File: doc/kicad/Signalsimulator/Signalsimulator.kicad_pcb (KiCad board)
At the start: 2 copper layers, 38.1 x 38.1 mm, 14 parts, among them J1 Conn_02x03_Odd_Even

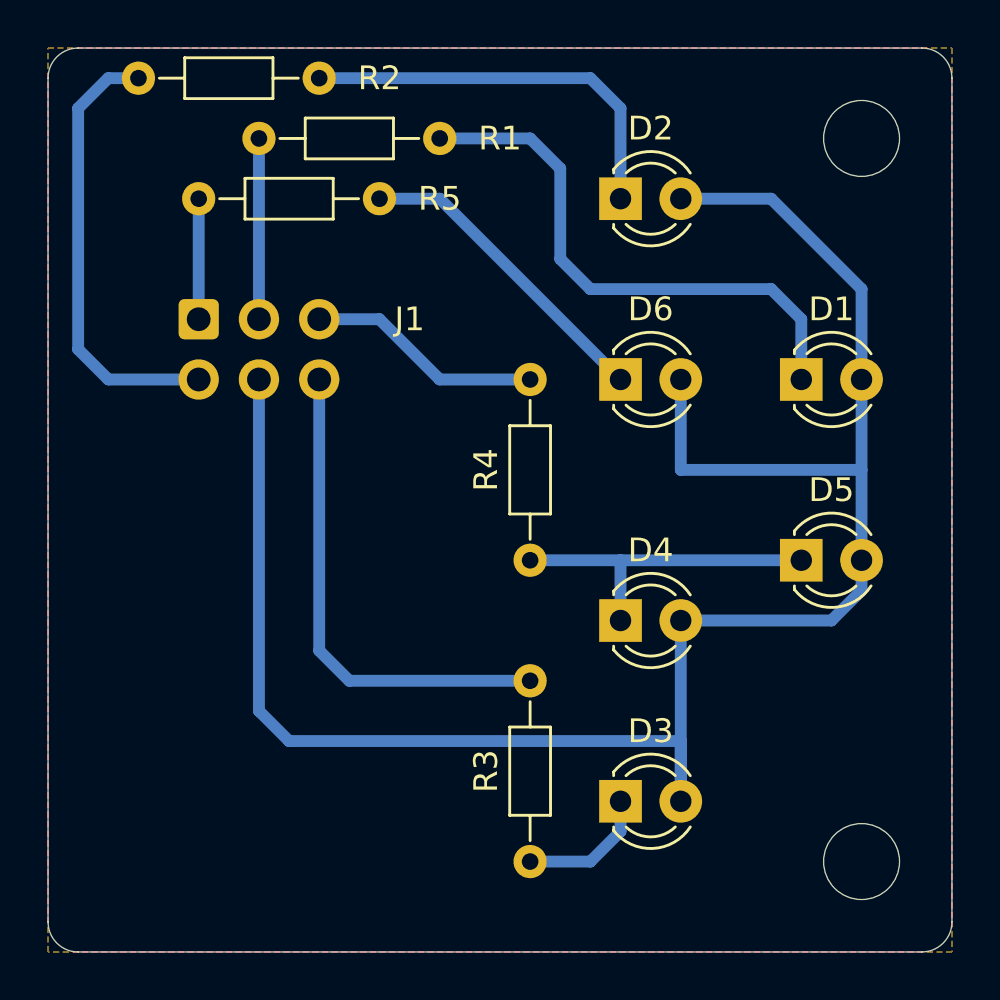
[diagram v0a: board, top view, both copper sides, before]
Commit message: Widerständer auf Rückseite, Widerstandswerte angepasst
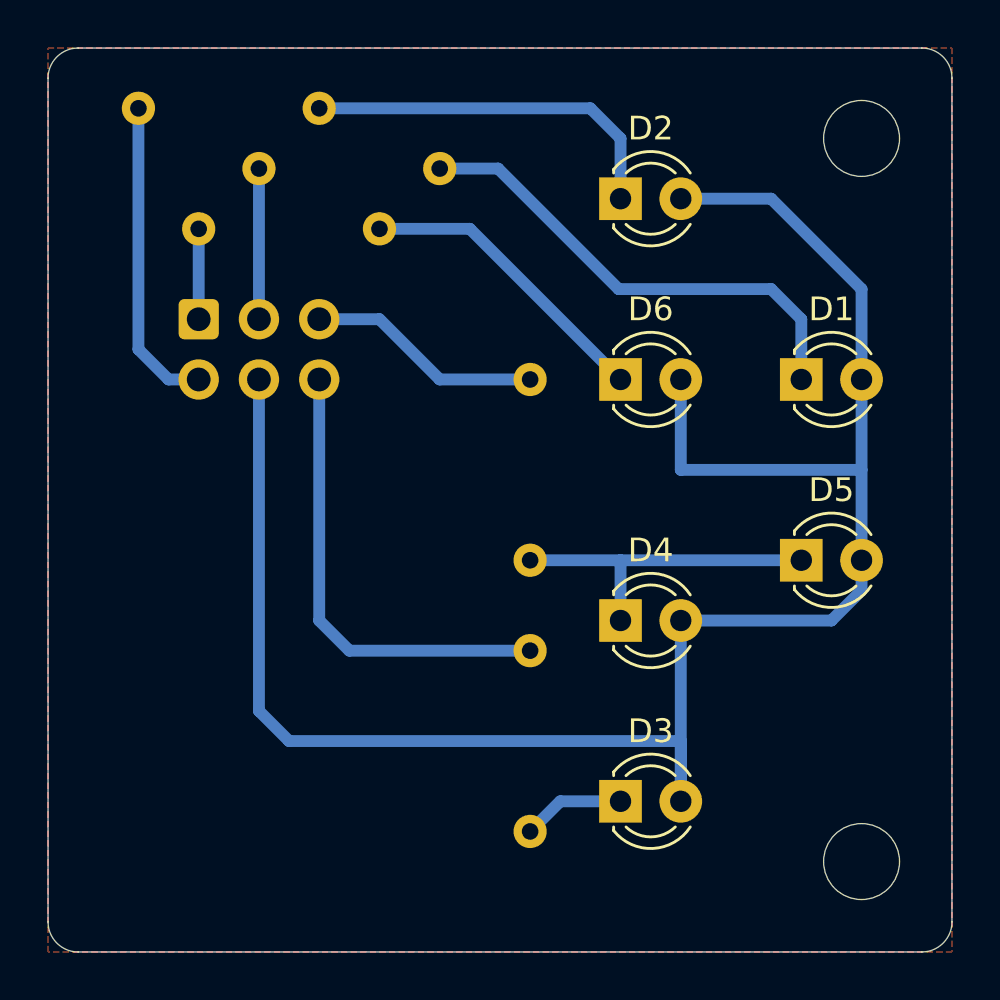
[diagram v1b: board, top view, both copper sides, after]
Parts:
- R1, R2, R3, R4, R5: moved to B.Cu
- moved R5 1.27 mm to (39.4, 33.0)
- moved R1 1.27 mm to (41.9, 30.5)
- moved R2 1.27 mm to (36.8, 27.9)
- moved R3 1.27 mm to (45.7, 58.4)
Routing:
- net Net-(J1-Pad2): track 18.8 -> 13.2 mm
- net Net-(D1-Pad1): track 23.2 -> 20.4 mm
- net Net-(J1-Pad1): track 5.08 -> 3.81 mm
- net Net-(J1-Pad6): track 20.8 -> 19.6 mm
- net Net-(J1-Pad3): track 7.62 -> 6.35 mm
- net Net-(D2-Pad1): track 17.0 -> 15.8 mm
- net Net-(D3-Pad1): track 5.61 -> 4.34 mm
- net Net-(D6-Pad1): track 13.3 -> 12.8 mm
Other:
- board text added: "HL-Signal v1.1"
- board text added: "©H3-H5N6 2022"
- board text removed: "©H3-H5N6 2021 HL-Signal v1.0"
